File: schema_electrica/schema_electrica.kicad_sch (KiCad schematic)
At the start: 13 parts, among them M1 Motor_DC, M2 Motor_DC, M3 Motor_DC, M4 Motor_DC, SW1 SW_DIP_x01, U1 L298N, U2 DHT11

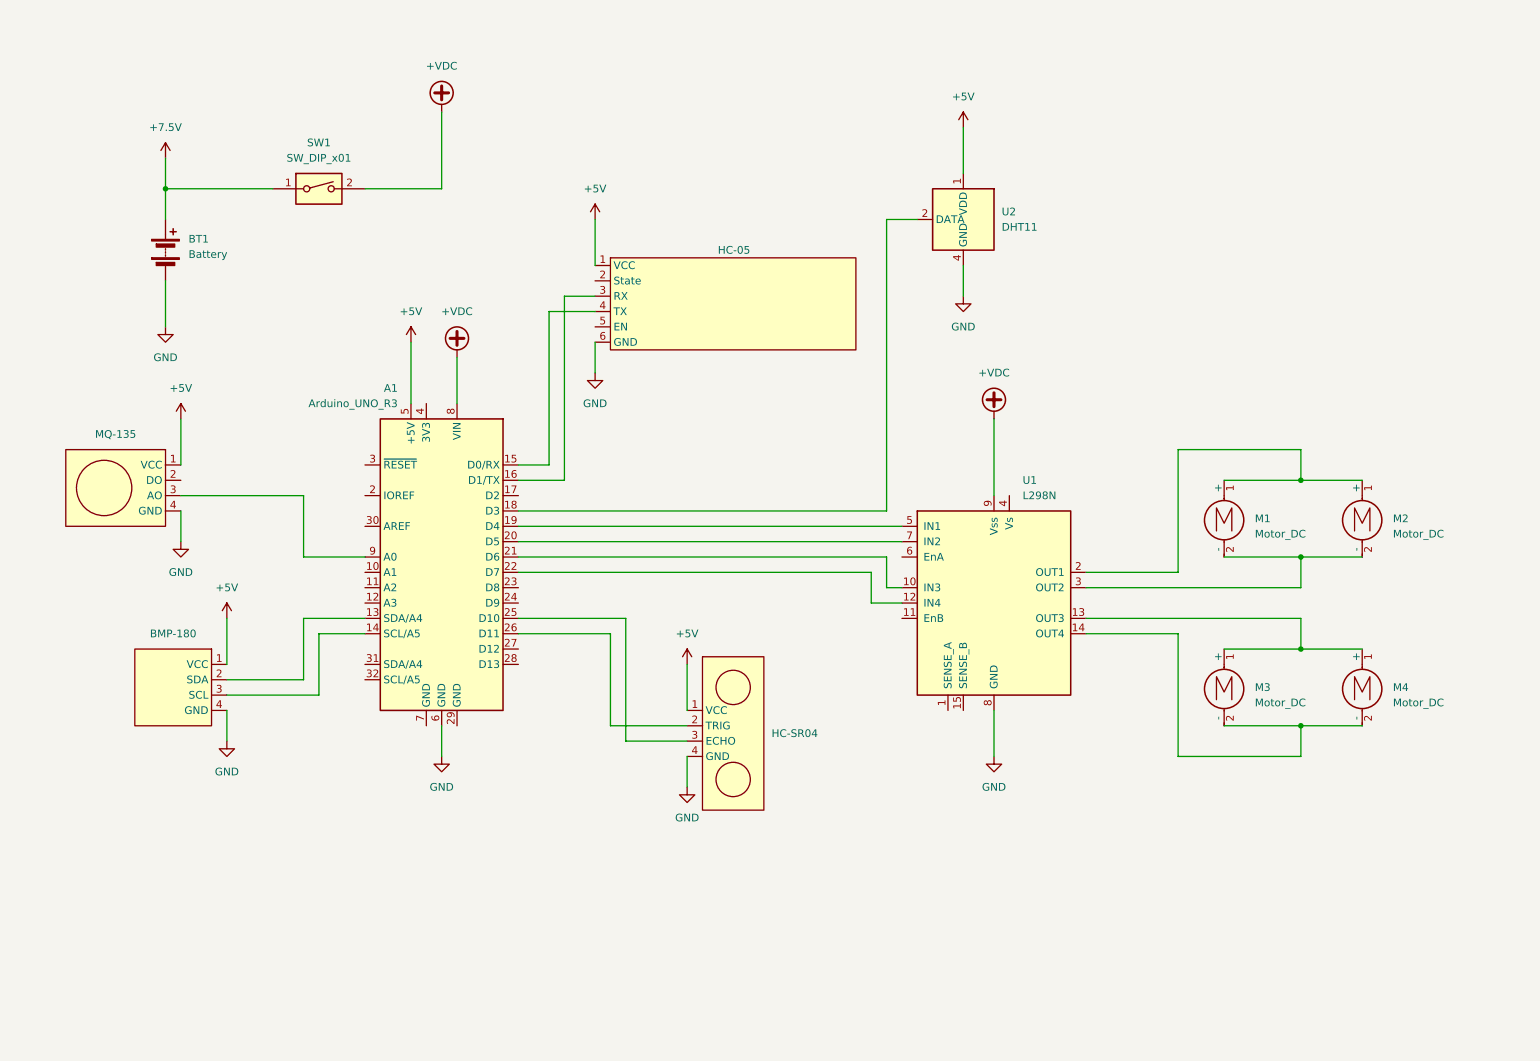
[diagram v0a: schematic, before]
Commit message: actualizare schema
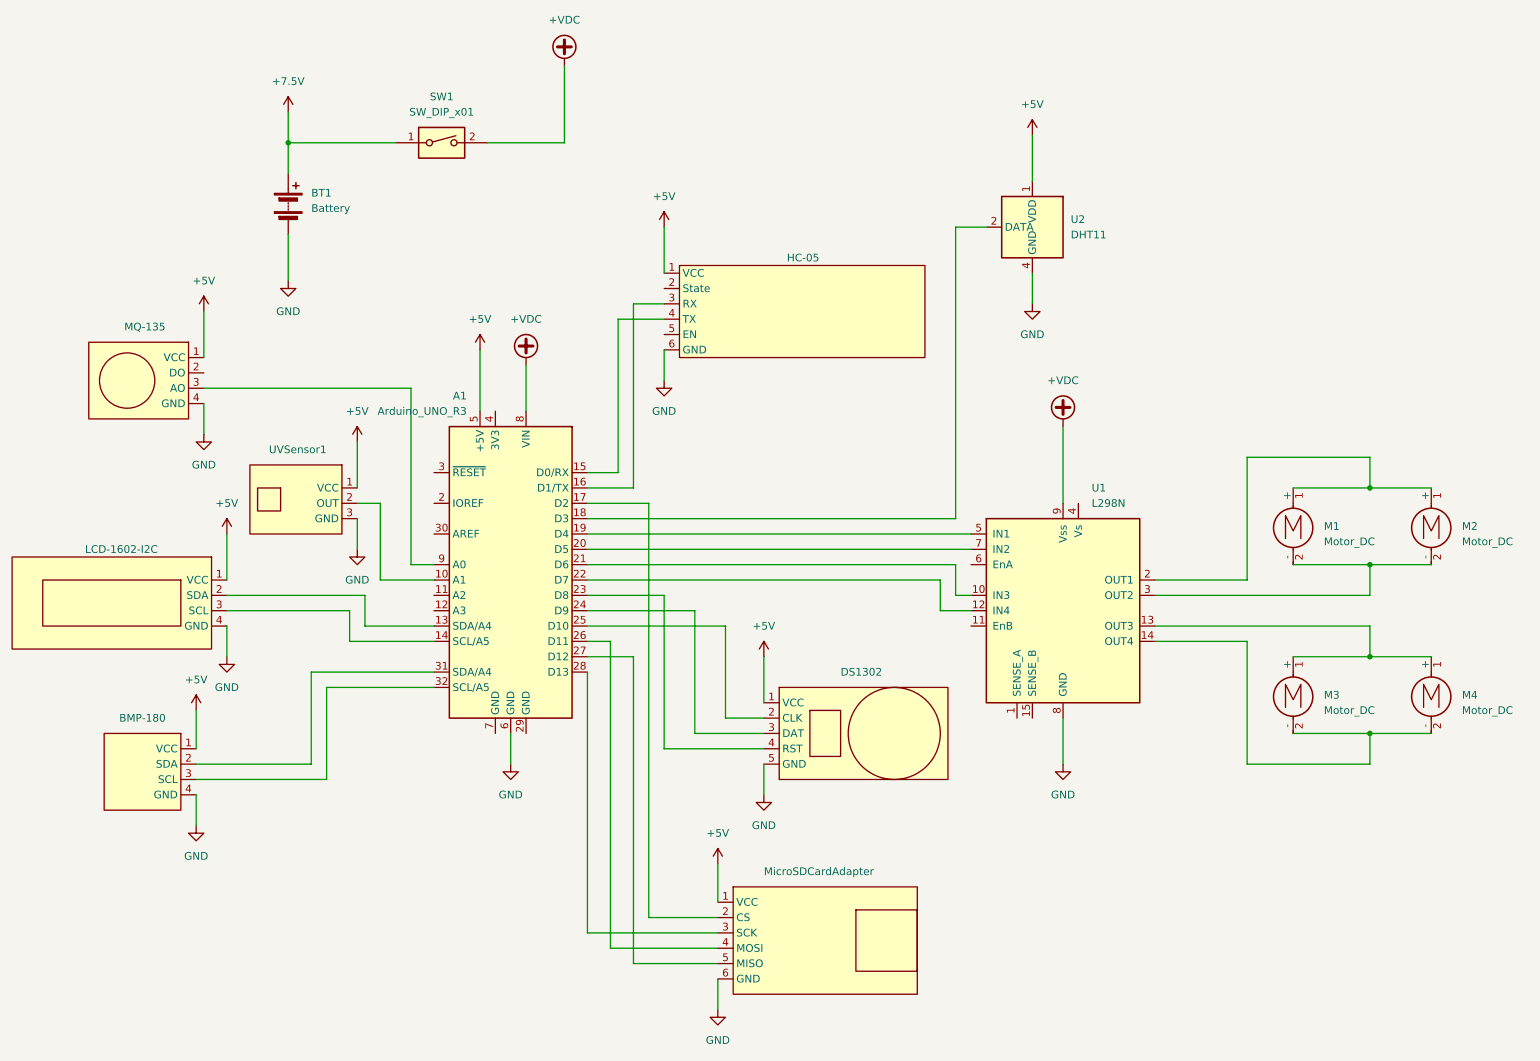
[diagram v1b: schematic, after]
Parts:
- removed HC-SR04: ~, symbol Arduino_Components:HC-SR04
- removed MQ-135: ~, symbol Arduino_Components:MQ-135
- added DS1302: ~, symbol ArduinoComponents:DS1302
- added LCD-1602-I2C: ~, symbol ArduinoComponents:LCD_1602_I2C
- added MQ-135: ~, symbol ArduinoComponents:MQ-135
- added MicroSDCardAdapter: ~, symbol ArduinoComponents:Micro_SD_Card_Adapter
- added UVSensor1: ~, symbol ArduinoComponents:UV_Sensor
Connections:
- net +5V: now also DS1302.1 (VCC), LCD-1602-I2C.1 (VCC), MQ-135.1 (VCC), MicroSDCardAdapter.1 (VCC), UVSensor1.1 (VCC)
- net GND: now also DS1302.5 (GND), LCD-1602-I2C.4 (GND), MQ-135.4 (GND), MicroSDCardAdapter.6 (GND), UVSensor1.3 (GND)
- net at A1.26 (D11): now also MicroSDCardAdapter.4 (MOSI)
- net at A1.25 (D10): now also DS1302.2 (CLK)
- net at A1.9 (A0): now also MQ-135.3 (AO)
- net at A1.13 (SDA/A4): now also LCD-1602-I2C.2 (SDA); no longer BMP-180.2 (SDA)
- net at A1.14 (SCL/A5): now also LCD-1602-I2C.3 (SCL); no longer BMP-180.3 (SCL)
- net at A1.10 (A1): now also UVSensor1.2 (OUT)
- net at A1.17 (D2): now also MicroSDCardAdapter.2 (CS)
- net at A1.23 (D8): now also DS1302.4 (RST)
- net at A1.24 (D9): now also DS1302.3 (DAT)
- net at A1.27 (D12): now also MicroSDCardAdapter.5 (MISO)
- net at A1.28 (D13): now also MicroSDCardAdapter.3 (SCK)
- net at A1.31 (SDA/A4): now also BMP-180.2 (SDA)
- net at A1.32 (SCL/A5): now also BMP-180.3 (SCL)
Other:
- moved on the sheet: A1, BMP-180, BT1, HC-05, M1, M2, M3, M4, SW1, U1, U2
